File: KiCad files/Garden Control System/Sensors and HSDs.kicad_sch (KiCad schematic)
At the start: 25 parts, among them U3 UCC27624DR, U4 INA4180A2IPWR, U5 UCC27624DR, U6 IRLML6344TRPBF, U7 IRLML6344TRPBF, U8 IRLML6344TRPBF

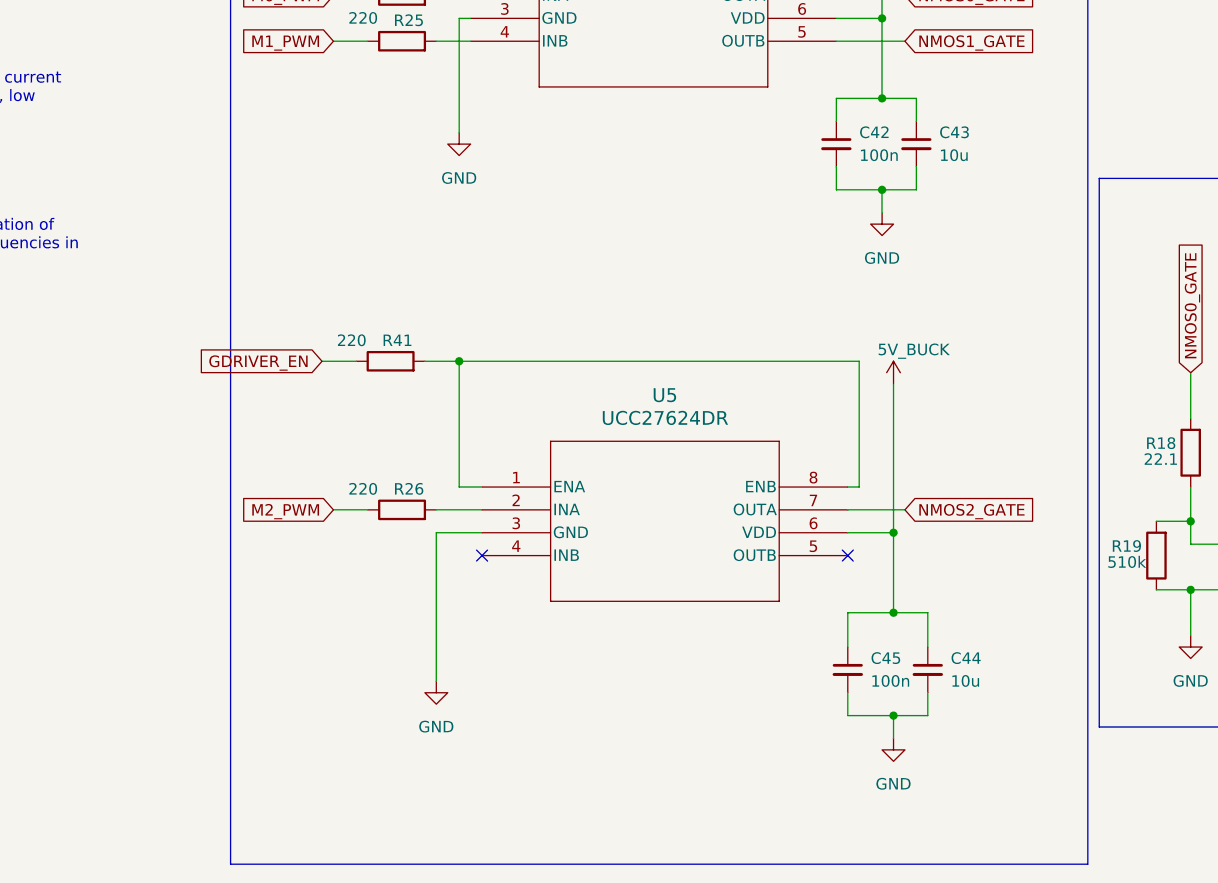
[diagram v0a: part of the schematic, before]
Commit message: saving changes
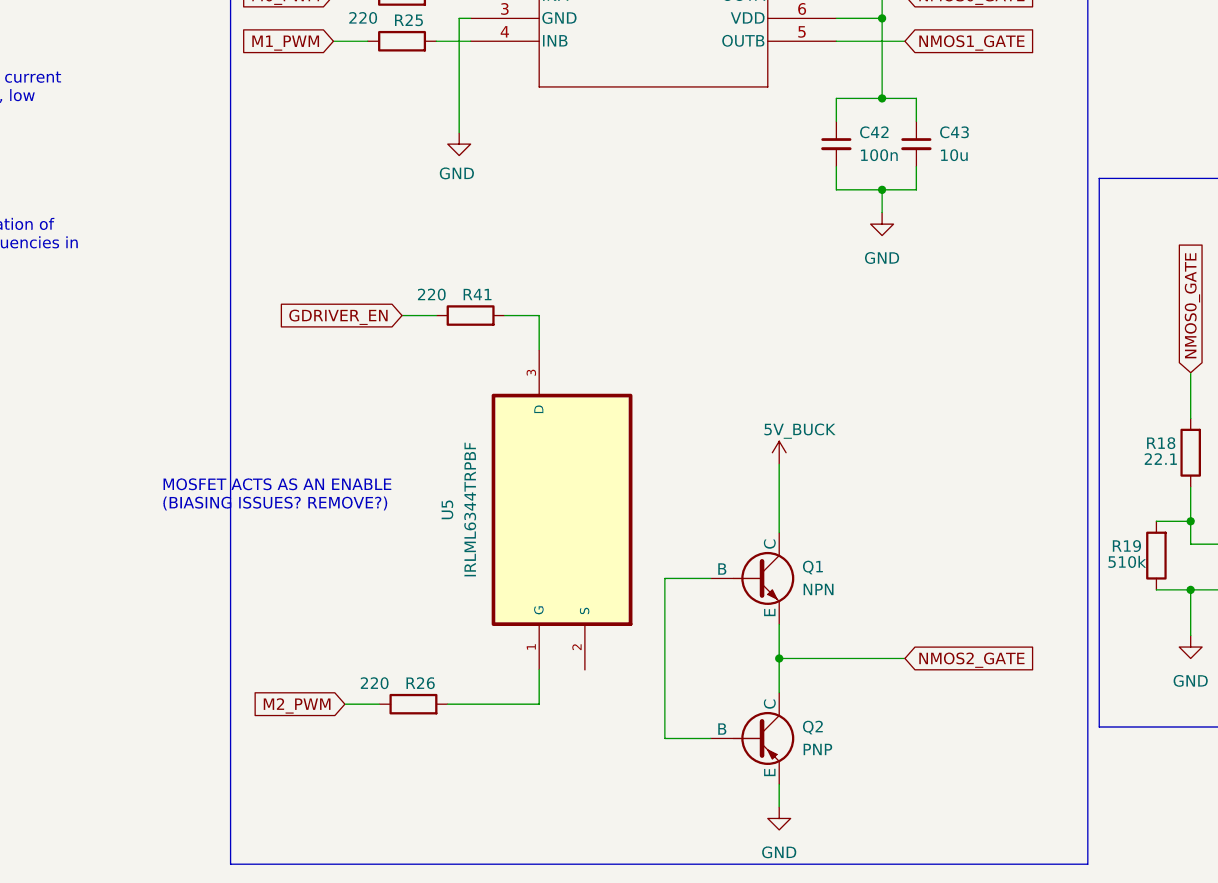
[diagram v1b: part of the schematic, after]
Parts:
- removed C44: 10u, symbol Device:C_Small
- removed C45: 100n, symbol Device:C_Small
- removed U5: UCC27624DR, SOIC_D0008A_TEX, symbol UCC27624DR:UCC27624DR
- added Q1: NPN, symbol Simulation_SPICE:NPN
- added Q2: PNP, symbol Simulation_SPICE:PNP
- added U5: IRLML6344TRPBF, IRLML6344TRPBF:SOT95P240X112-3N, symbol IRLML6344TRPBF:IRLML6344TRPBF
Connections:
- net 5V_BUCK: now also Q1.1 (C)
- net GND: now also Q2.3 (E)
- net NMOS2_GATE: now also Q1.3 (E), Q2.1 (C)
- net at R41.2: now also U5.3 (D)
- net at R26.2: now also U5.1 (G)
- new net: Q1.2 (B), Q2.2 (B)
- no-connect marks 2 -> 0
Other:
- note added: "MOSFET ACTS AS AN ENABLE (BIASING ISSUES? REMOVE?)"
- moved on the sheet: R26, R41
